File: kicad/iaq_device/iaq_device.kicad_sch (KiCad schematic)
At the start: 18 parts, among them J1 External Pins, SW1 B3S-1000, SW2 CO2 CAL, U1 WeMos_D1_mini_ESP32, U2 PMS7003, U3 SSD1306, U4 BME280, U5 MH-Z19, U6 SGP30, U7 TSL2561T

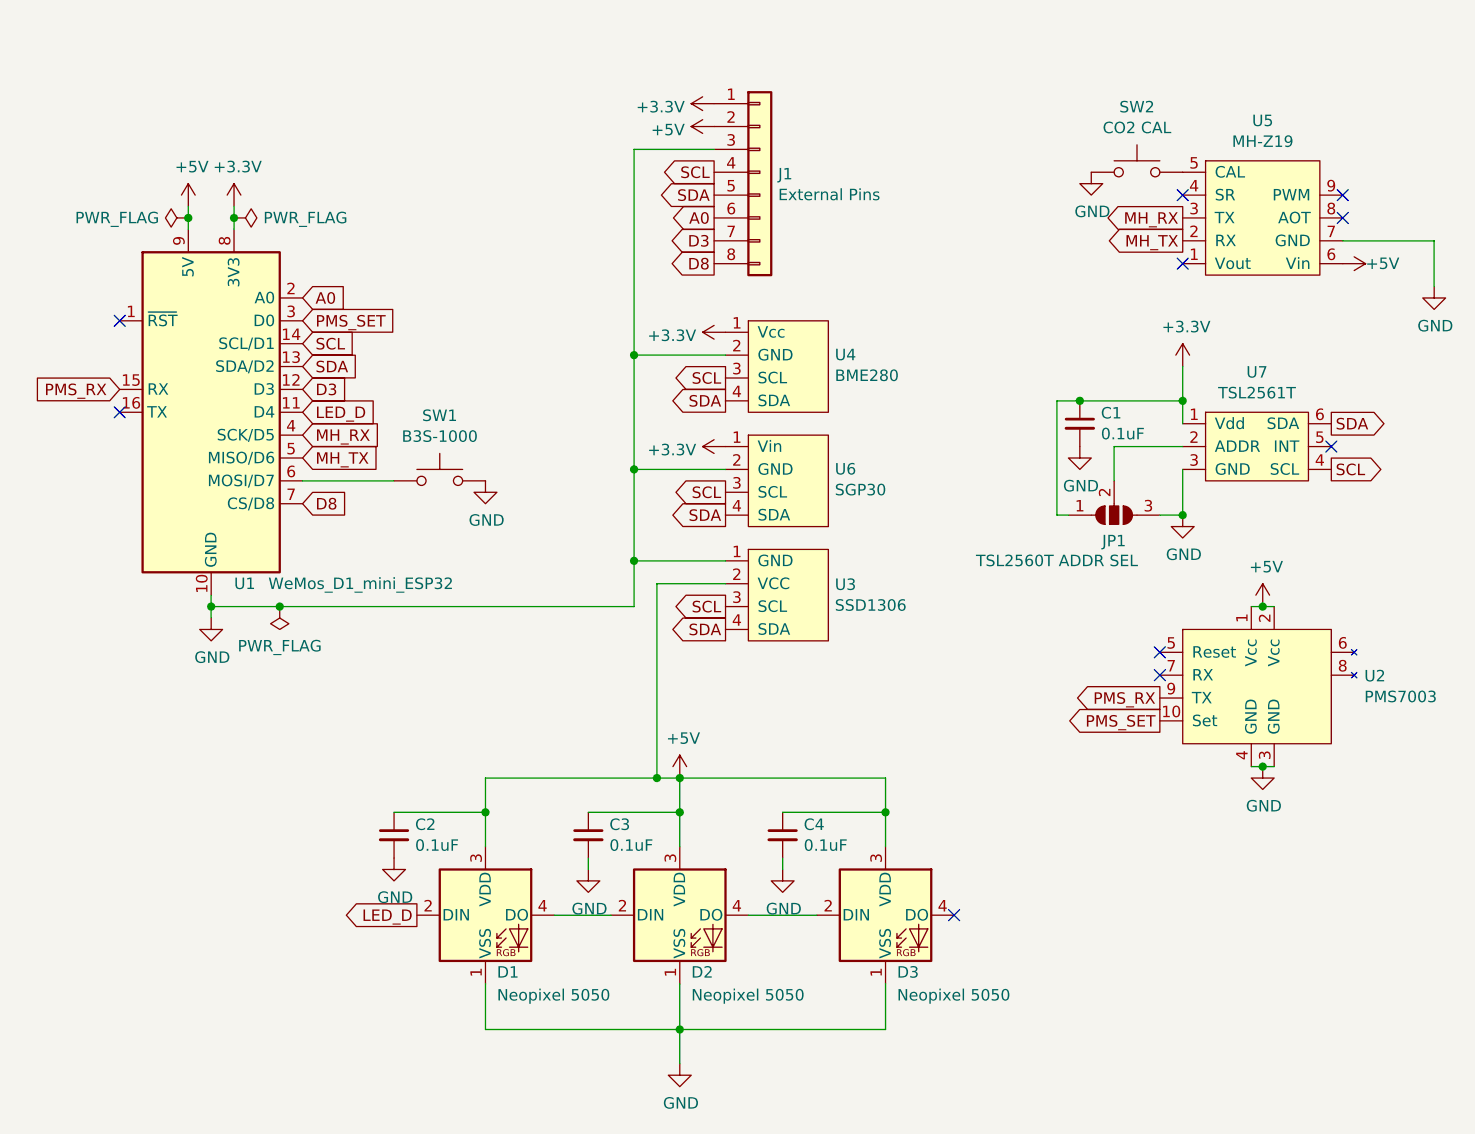
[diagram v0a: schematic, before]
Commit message: lots of changes
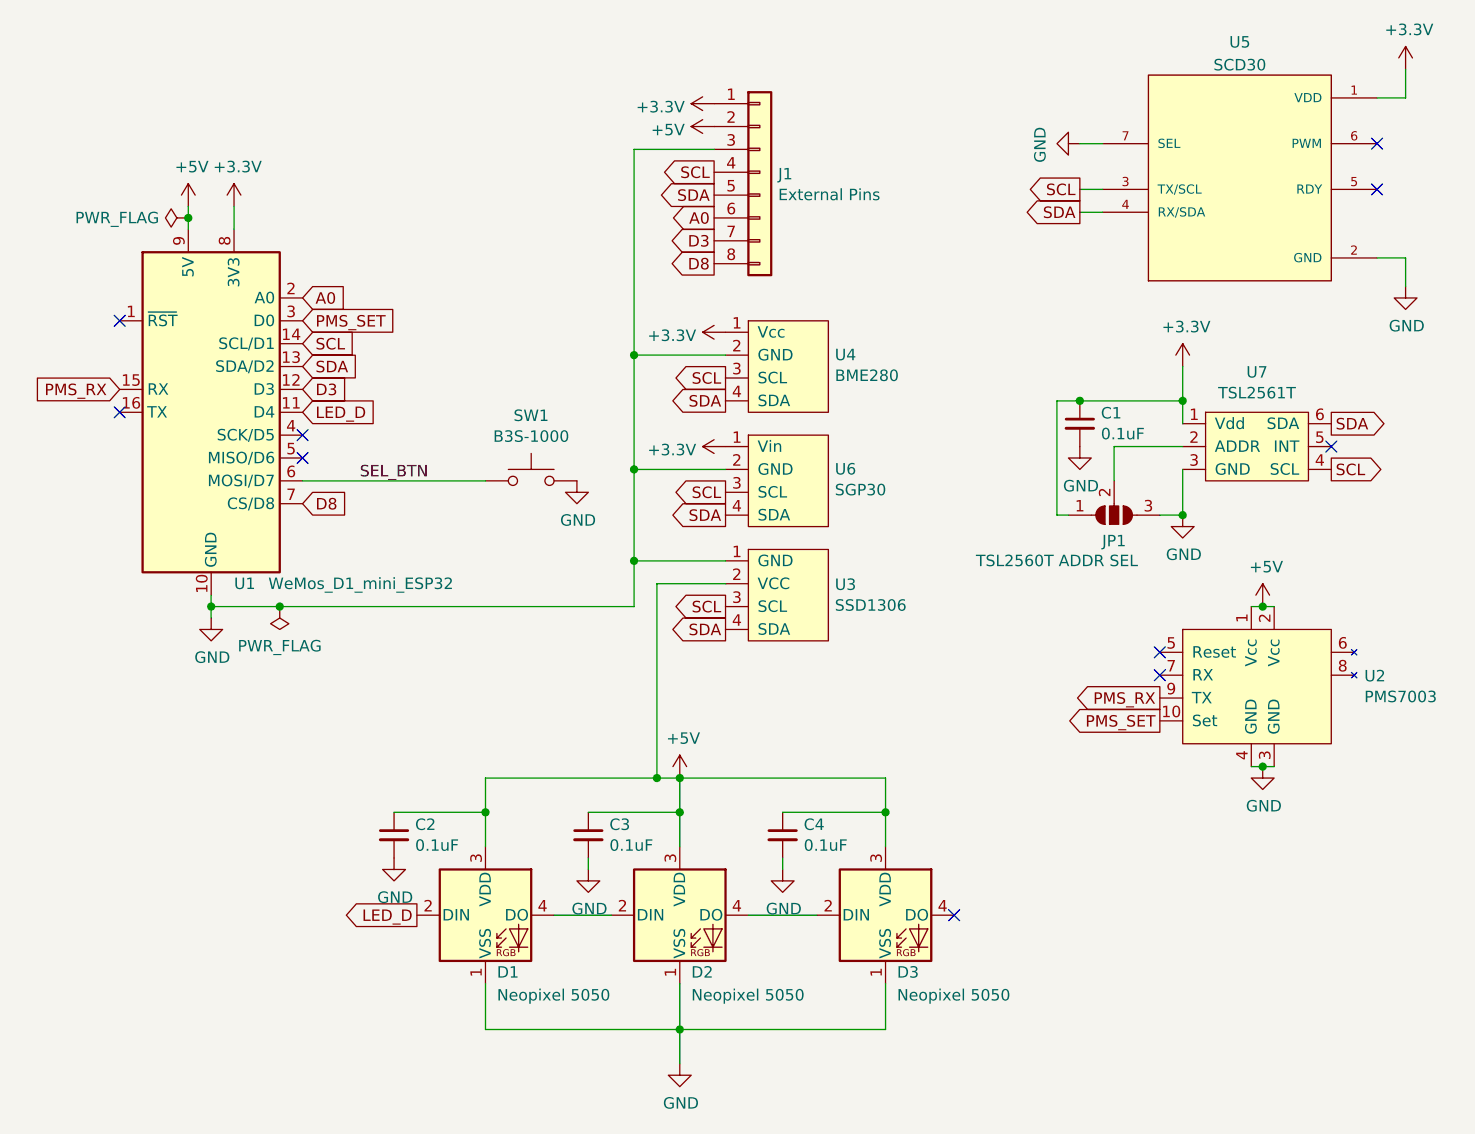
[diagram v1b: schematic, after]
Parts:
- removed SW2: CO2 CAL, Button_Switch_SMD:SW_SPST_B3U-1000P, symbol Switch:SW_Push
- removed U5: MH-Z19, iaq_board:MH-Z19, symbol iaq_board:MH-Z19
- added U5: SCD30, iaq_board:SCD30, symbol iaq_board:SCD30
- JP1: symbol iaq_device-rescue:SolderJumper_3_Open-Jumper -> Jumper:SolderJumper_3_Open
- U1: footprint iaq_board:WEMOS_D1_surface -> Module:WEMOS_D1_mini_light
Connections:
- net GND: now also U5.2 (GND), U5.7 (SEL)
- net SCL: now also U5.3 (TX/SCL)
- net SDA: now also U5.4 (RX/SDA)
- net SEL_BTN: now reaches SW1.1, U1.6 (MOSI/D7)
- net +3V3 renamed +3.3V
- net +3.3V: now also U5.1 (VDD)
- net MH_RX: no longer names the net of U1.4 (SCK/D5)
- net MH_TX: no longer names the net of U1.5 (MISO/D6)
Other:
- moved on the sheet: SW1

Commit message: changed co2 sensor to scd30 and rerouted the board
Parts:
- U1: footprint Module:WEMOS_D1_mini_light -> iaq_board:WEMOS_D1_surface
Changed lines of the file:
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@@
       (effects (font (size 1.27 1.27)) (justify left))
     )
-    (property "Footprint" "Module:WEMOS_D1_mini_light" (at 62.23 105.41 0)
+    (property "Footprint" "iaq_board:WEMOS_D1_surface" (at 62.23 105.41 0)
       (effects (font (size 1.27 1.27)) hide)
     )
